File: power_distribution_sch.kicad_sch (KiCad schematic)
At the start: 2 parts

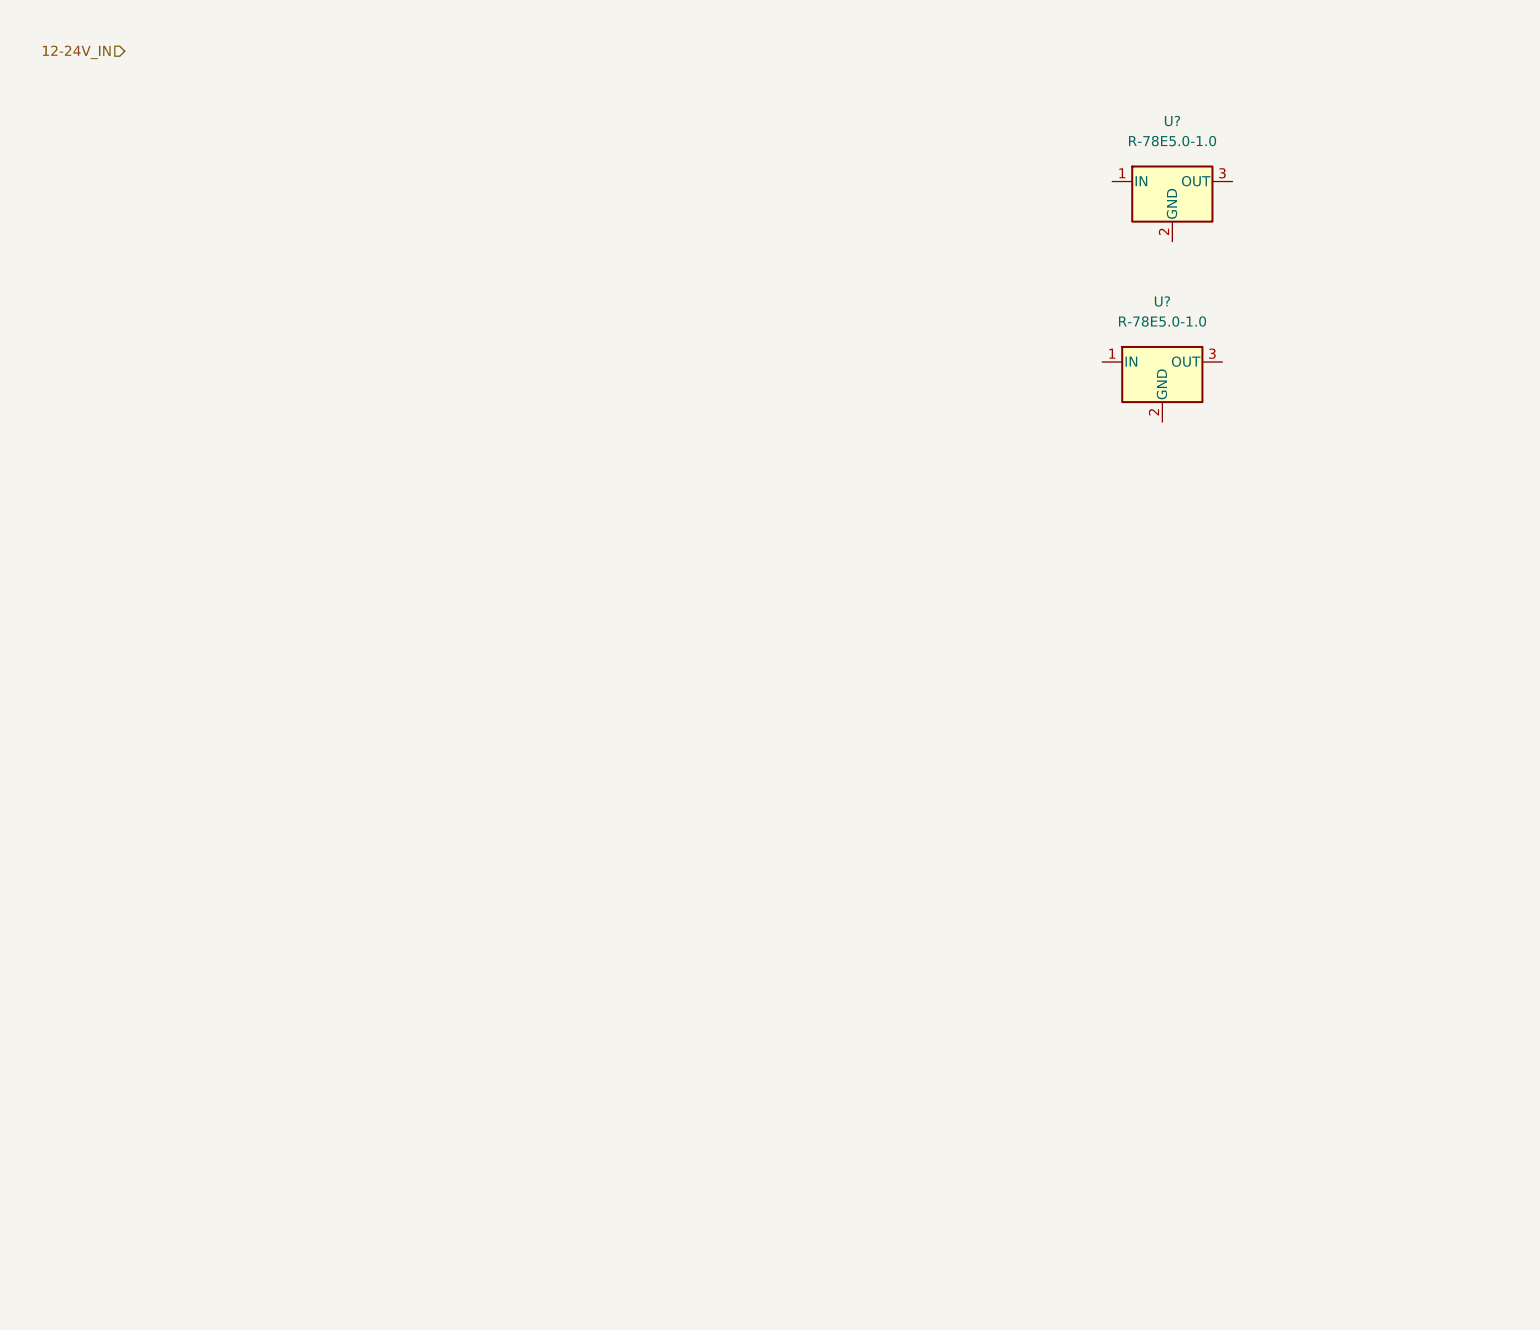
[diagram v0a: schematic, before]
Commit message: daily update
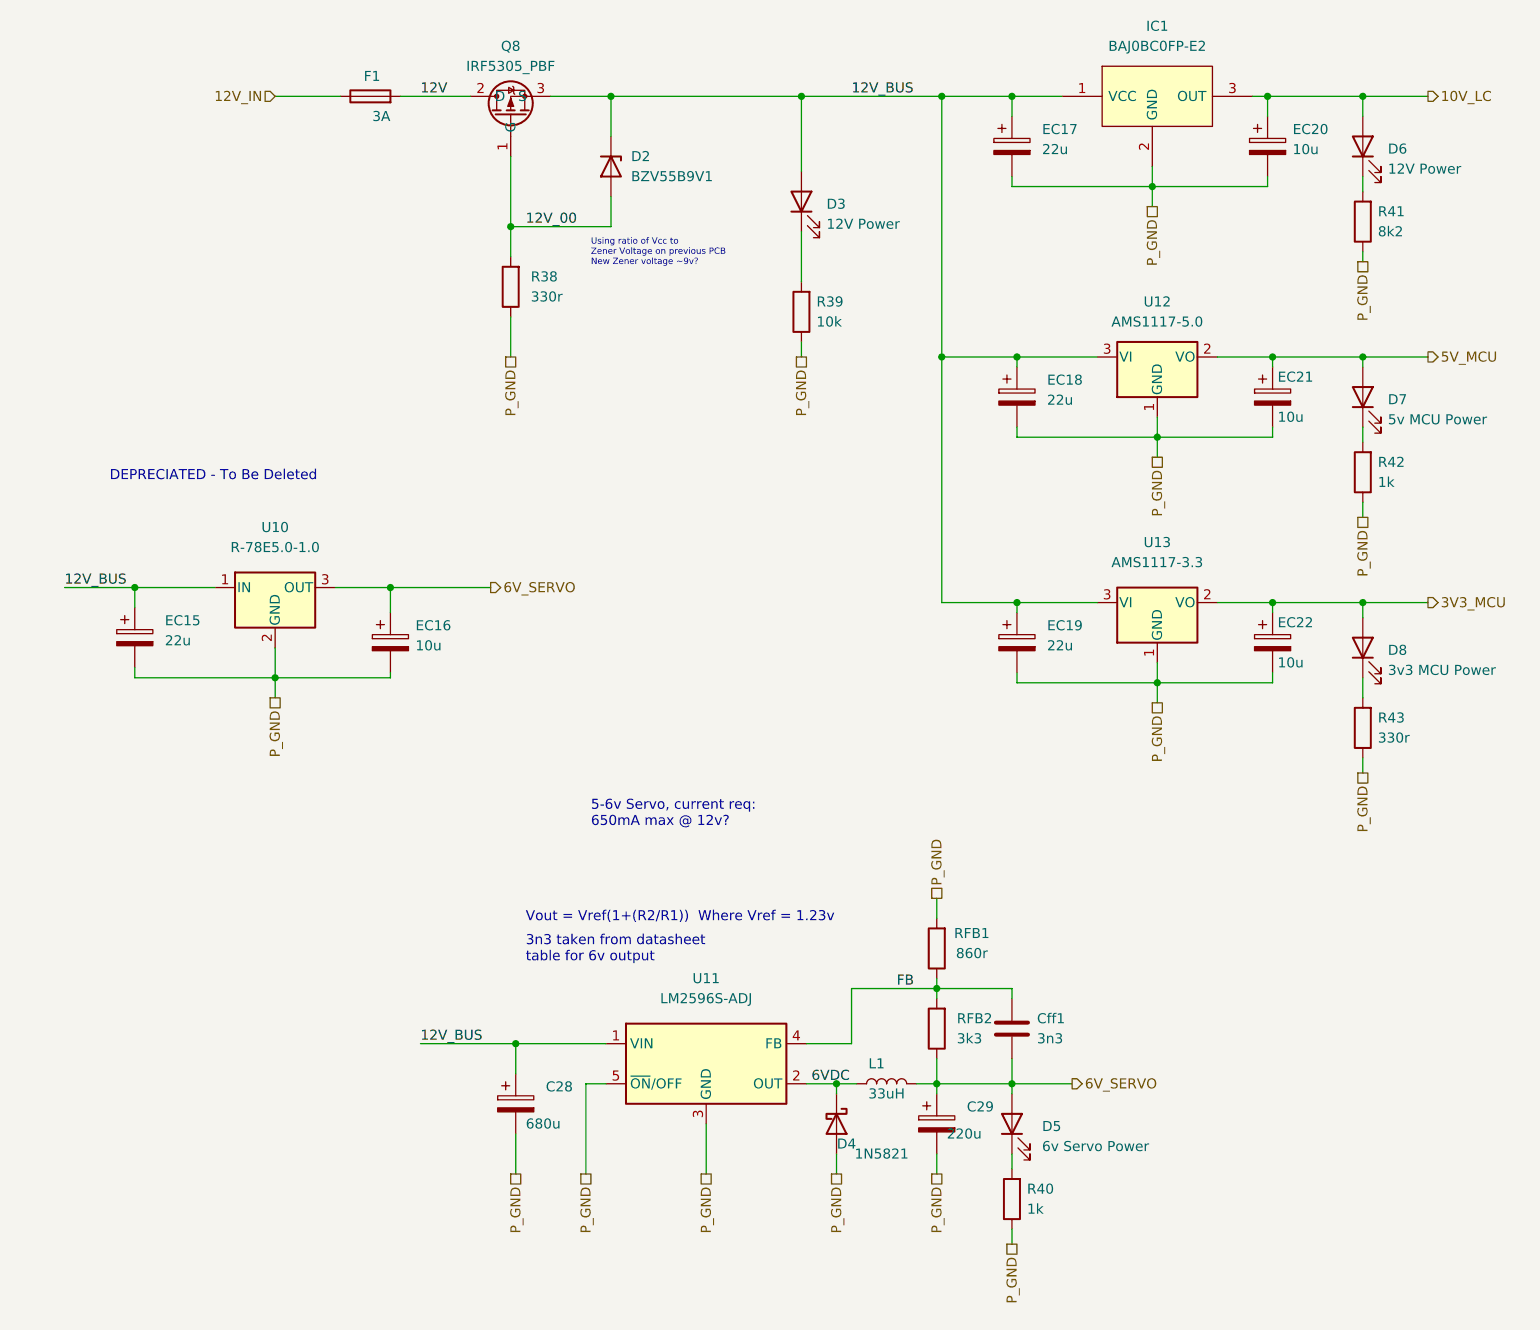
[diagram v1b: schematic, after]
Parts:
- removed U? (x2): R-78E5.0-1.0, Converter_DCDC:Converter_DCDC_RECOM_R-78E-0.5_THT, symbol Regulator_Switching:R-78E5.0-1.0
- added C28: 680u, Capacitor_THT:C_Radial_D12.5mm_H20.0mm_P5.00mm, symbol 000_Capacitor_Electrolytic_Immo:100u
- added C29: 220u, Capacitor_SMD:CP_Elec_6.3x7.7, symbol 000_Capacitor_Electrolytic_Immo:100u
- added Cff1: 3n3, Capacitor_SMD:C_0805_2012Metric_Pad1.18x1.45mm_HandSolder, symbol 000_Capacitor_Film_Immo:cap_film_0805
- added D2: BZV55B9V1, Diode_SMD:D_MiniMELF, symbol Diode:BZV55B9V1
- added D3, D6: 12V Power, Diode_SMD:D_0805_2012Metric_Pad1.15x1.40mm_HandSolder, symbol 000_Diodes_Immo:LED_0805_smd
- added D4: 1N5821, Diode_SMD:D_SMA, symbol Diode:1N5821
- added D5: 6v Servo Power, Diode_SMD:D_0805_2012Metric_Pad1.15x1.40mm_HandSolder, symbol 000_Diodes_Immo:LED_0805_smd
- added D7: 5v MCU Power, Diode_SMD:D_0805_2012Metric_Pad1.15x1.40mm_HandSolder, symbol 000_Diodes_Immo:LED_0805_smd
- added D8: 3v3 MCU Power, Diode_SMD:D_0805_2012Metric_Pad1.15x1.40mm_HandSolder, symbol 000_Diodes_Immo:LED_0805_smd
- added EC15, EC17, EC18, EC19: 22u, Capacitor_SMD:CP_Elec_6.3x5.9, symbol 000_Capacitor_Electrolytic_Immo:22u
- added EC16, EC20, EC21, EC22: 10u, Capacitor_SMD:CP_Elec_6.3x5.9, symbol 000_Capacitor_Electrolytic_Immo:22u
- added F1: 3A, Fuse:Fuseholder_Cylinder-5x20mm_Stelvio-Kontek_PTF78_Horizontal_Open, symbol 000_Protection_Immo:Fuse
- added IC1: BAJ0BC0FP-E2, Package_TO_SOT_SMD:TO-252-2, symbol SamacSys_Parts:BAJ0BC0FP-E2
- added L1: 33uH, Inductor_SMD:L_12x12mm_H8mm, symbol Device:L
- added Q8: IRF5305_PBF, Package_TO_SOT_THT:TO-220-3_Vertical, symbol 000_MOSFET_Immo:IRF5305_PBF
- added R38, R43: 330r, Resistor_SMD:R_0805_2012Metric_Pad1.20x1.40mm_HandSolder, symbol 000_Resistors_Immo:Resistor_0805
- added R39: 10k, Resistor_SMD:R_0805_2012Metric_Pad1.20x1.40mm_HandSolder, symbol 000_Resistors_Immo:Resistor_0805
- added R40, R42: 1k, Resistor_SMD:R_0805_2012Metric_Pad1.20x1.40mm_HandSolder, symbol 000_Resistors_Immo:Resistor_0805
- added R41: 8k2, Resistor_SMD:R_0805_2012Metric_Pad1.20x1.40mm_HandSolder, symbol 000_Resistors_Immo:Resistor_0805
- added RFB1: 860r, Resistor_SMD:R_0805_2012Metric_Pad1.20x1.40mm_HandSolder, symbol 000_Resistors_Immo:Resistor_0805
- added RFB2: 3k3, Resistor_SMD:R_0805_2012Metric_Pad1.20x1.40mm_HandSolder, symbol 000_Resistors_Immo:Resistor_0805
- added U10: R-78E5.0-1.0, Converter_DCDC:Converter_DCDC_RECOM_R-78E-0.5_THT, symbol Regulator_Switching:R-78E5.0-1.0
- added U11: LM2596S-ADJ, Package_TO_SOT_SMD:TO-263-5_TabPin3, symbol Regulator_Switching:LM2596S-ADJ
- added U12: AMS1117-5.0, Package_TO_SOT_SMD:SOT-223-3_TabPin2, symbol Regulator_Linear:AMS1117-5.0
- added U13: AMS1117-3.3, Package_TO_SOT_SMD:SOT-223-3_TabPin2, symbol Regulator_Linear:AMS1117-3.3
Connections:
- new net: D3.1 (K), R39.2
- new net: D8.1 (K), R43.2
- new net: D6.1 (K), R41.2
- new net: D7.1 (K), R42.2
- new net: D5.1 (K), R40.2
- new net 10V_LC: D6.2 (A), EC20.1, IC1.3 (OUT)
- new net 12V: F1.2, Q8.2 (D)
- new net 12V_00: D2.2 (A), Q8.1 (G), R38.2
- new net 12V_BUS: C28.1, D2.1 (K), D3.2 (A), EC15.1, EC17.1, EC18.1, EC19.1, IC1.1 (VCC), Q8.3 (S), U10.1 (IN), U11.1 (VIN), U12.3 (VI), U13.3 (VI)
- new net 12V_IN: F1.1
- new net 3V3_MCU: D8.2 (A), EC22.1, U13.2 (VO)
- new net 5V_MCU: D7.2 (A), EC21.1, U12.2 (VO)
- new net 6VDC: D4.1 (K), L1.1, U11.2 (OUT)
- new net 6V_SERVO: C29.1, Cff1.2, D5.2 (A), EC16.1, L1.2, RFB2.1, U10.3 (OUT)
- new net FB: Cff1.1, RFB1.1, RFB2.2, U11.4 (FB)
- new net P_GND: C28.2, C29.2, D4.2 (A), EC15.2, EC16.2, EC17.2, EC18.2, EC19.2, EC20.2, EC21.2, EC22.2, IC1.2 (GND), R38.1, R39.1, R40.1, R41.1, R42.1, R43.1, RFB1.2, U10.2 (GND), U11.3 (GND), U11.5 (~{ON}/OFF), U12.1 (GND), U13.1 (GND)
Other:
- note added: "3n3 taken from datasheet table for 6v output"
- note added: "5-6v Servo, current req: 650mA max @ 12v?"
- note added: "DEPRECIATED - To Be Deleted"
- note added: "Using ratio of Vcc to Zener Voltage on previous PCB New Zener voltage ~9v?"
- note added: "Vout = Vref(1+(R2/R1)) Where Vref = 1.23v"
